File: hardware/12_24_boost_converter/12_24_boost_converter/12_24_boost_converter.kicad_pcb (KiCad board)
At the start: 2 copper layers, 45.5 x 48.5 mm, 18 parts, among them J1 Conn_01x02, J2 Conn_01x02, J3 Conn_01x02, Q1 IRFZ24NPBF, U1 LM555xM

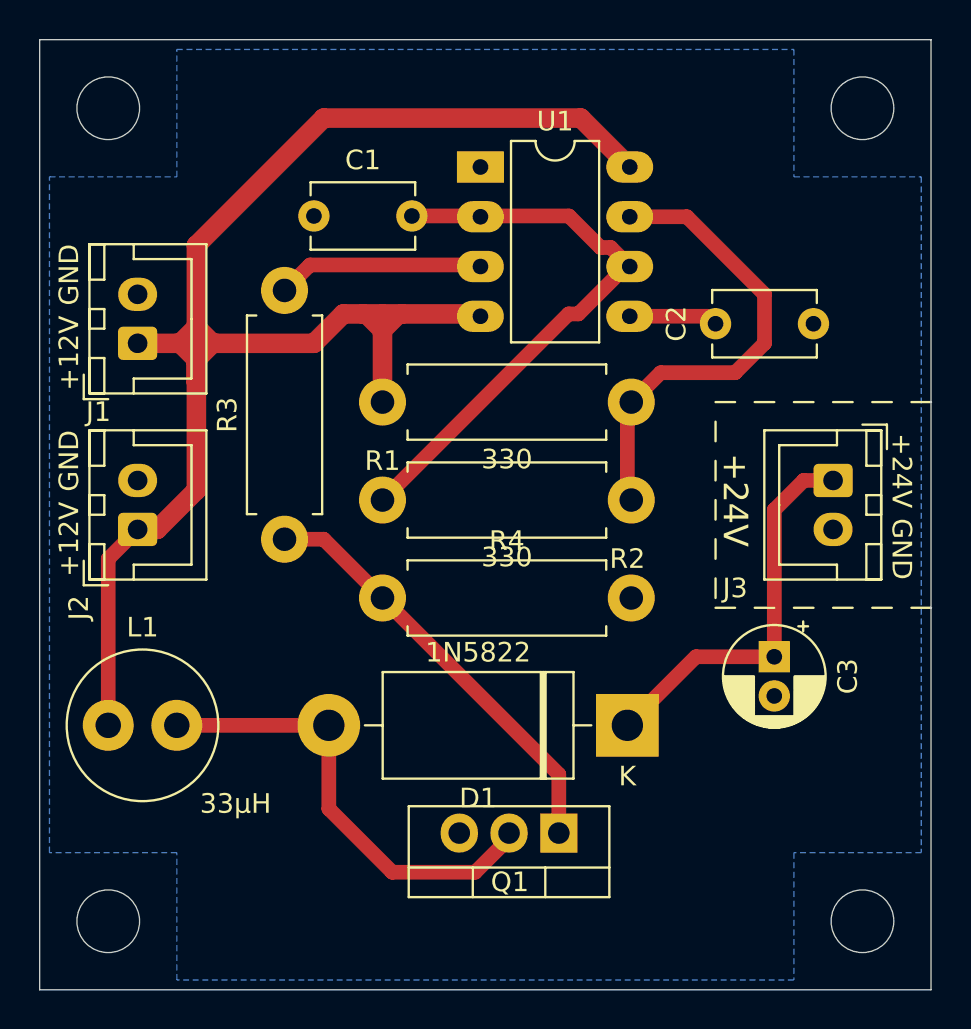
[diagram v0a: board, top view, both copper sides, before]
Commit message: Update boost converter
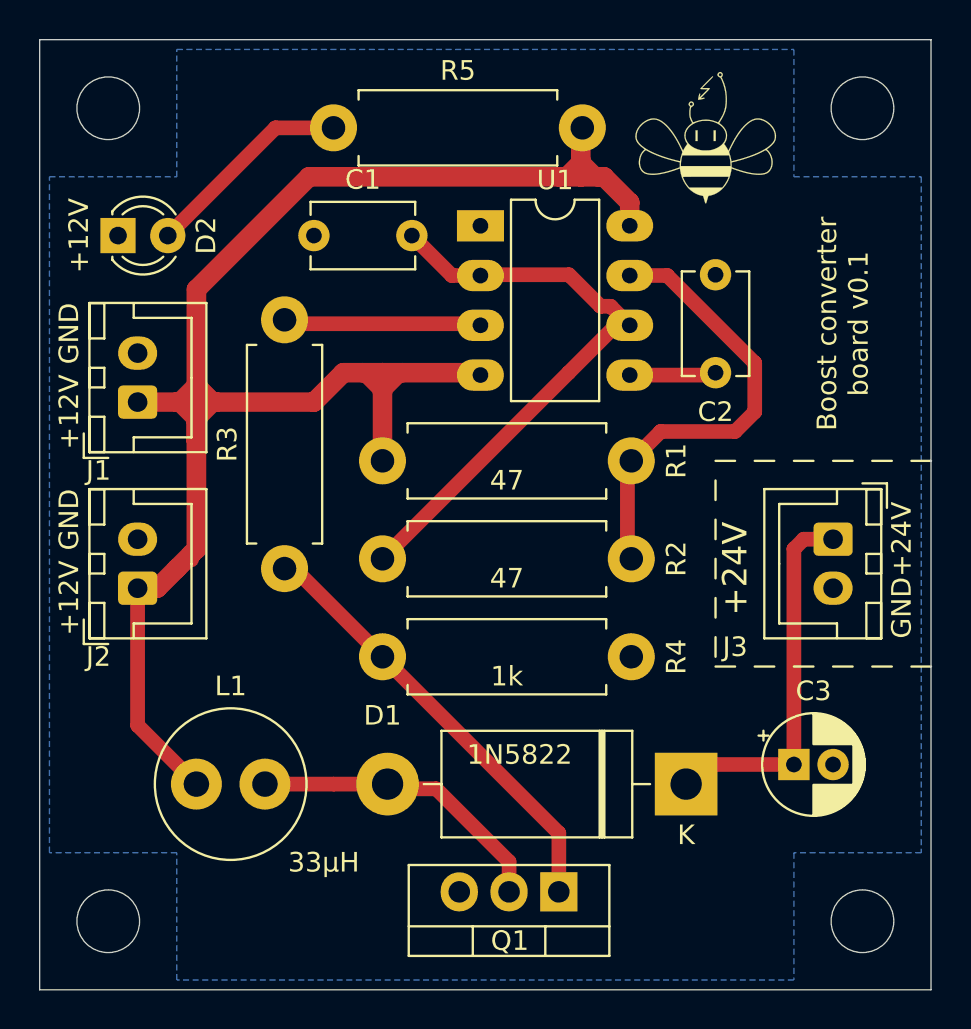
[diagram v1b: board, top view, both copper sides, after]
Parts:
- added D2: LED, LED_THT:LED_D3.0mm, F.Cu at (109.0, 90.0)
- added G***: LOGO, logo-beehive:logo-beehive-7_2х6_7mm, F.Cu at (139.0, 85.0)
- added R5: 560, Resistor_THT:R_Axial_DIN0411_L9.9mm_D3.6mm_P12.70mm_Horizontal, F.Cu at (120.0, 84.5)
- C1, C2: value 10nF -> 100nF
- R1, R2, R3: value 330 -> 47
- moved C2 5.59 mm to (139.5, 92.0), turned to 270 degrees
- moved C3 5.59 mm to (143.5, 117.0), turned to 0 degrees
- moved L1 5.41 mm to (113.0, 118.0)
- moved D1 4.24 mm to (138.0, 118.0)
- moved J1 3.00 mm to (110.0, 98.5)
- moved J2 3.00 mm to (110.0, 108.0)
- moved J3 3.00 mm to (145.5, 105.5)
- moved Q1 3.00 mm to (131.5, 123.5)
- moved R1 3.00 mm to (122.5, 101.5)
- moved R2 3.00 mm to (122.5, 106.5)
- moved R4 3.00 mm to (122.5, 111.5)
- moved U1 3.00 mm to (127.5, 89.5)
- moved R3 1.50 mm to (117.5, 107.0)
- moved C1 1.00 mm to (119.0, 90.0)
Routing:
- net Net-(D2-Pad2): track 0.00 -> 10.7 mm
- net +12V: track 86.8 -> 94.4 mm
- net Net-(D1-Pad2): track 23.3 -> 15.9 mm
- net Net-(R1-Pad2): track 24.2 -> 23.2 mm
- net Net-(C1-Pad2): track 29.8 -> 30.6 mm
- net Net-(Q1-Pad1): track 21.5 -> 22.1 mm
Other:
- board text added: "Boost converter board v0.1"
